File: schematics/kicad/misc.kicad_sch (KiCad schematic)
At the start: 41 parts, among them P4 DIN41612_03x32_C_Split

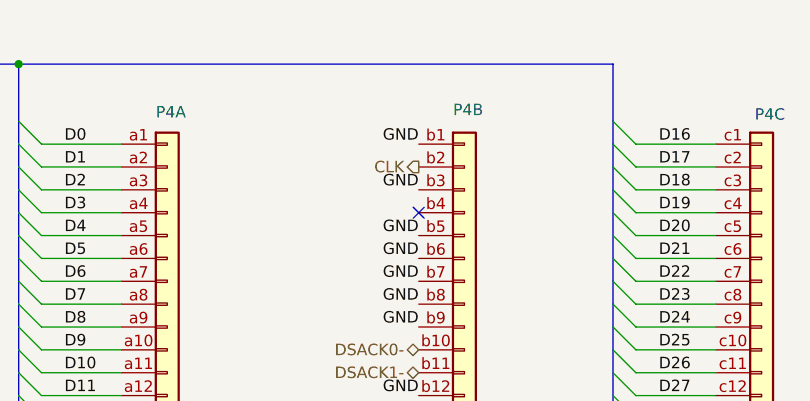
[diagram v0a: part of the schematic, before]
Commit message: Finish routing and misc fixes in the analog section
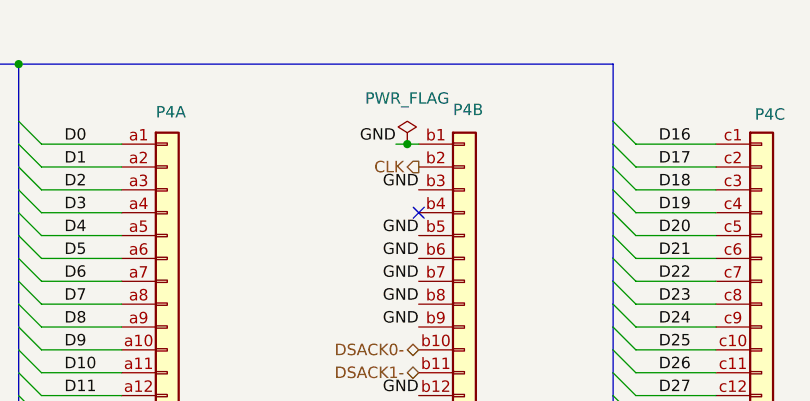
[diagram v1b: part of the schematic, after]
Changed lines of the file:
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@@
 	)
 	(junction
+		(at 208.28 45.72)
+		(diameter 0)
+		(color 0 0 0 0)
+	)
+	(junction
 		(at 73.66 38.1)
 		(diameter 0)
@@
 	(wire
 		(pts
+			(xy 207.01 45.72) (xy 208.28 45.72)
+		)
+		(stroke
+			(width 0)
+			(type default)
+		)
+	)
+	(wire
+		(pts
 			(xy 233.68 63.5) (xy 242.57 63.5)
 		)
@@
 	(wire
 		(pts
+			(xy 208.28 45.72) (xy 209.55 45.72)
+		)
+		(stroke
+			(width 0)
+			(type default)
+		)
+	)
+	(wire
+		(pts
 			(xy 233.68 71.12) (xy 242.57 71.12)
 		)
@@
 	)
 	(label "GND"
-		(at 209.55 45.72 180)
+		(at 207.01 45.72 180)
 		(effects
 			(font
@@
 					(unit 1)
 				)
+			)
+		)
+	)
+	(symbol
+		(lib_id "power:PWR_FLAG")
+		(at 208.28 45.72 0)
+		(unit 1)
+		(exclude_from_sim no)
+		(in_bom yes)
+		(on_board yes)
+		(dnp no)
+		(fields_autoplaced yes)
+		(property "Reference" "#FLG05"
+			(at 208.28 43.815 0)
+			(effects
+				(font
+					(size 1.27 1.27)
+				)
+				(hide yes)
+			)
+		)
+		(property "Value" "PWR_FLAG"
+			(at 208.28 40.64 0)
+			(effects
+				(font
+					(size 1.27 1.27)
+				)
+			)
+		)
+		(property "Footprint" ""
+			(at 208.28 45.72 0)
+			(effects
+				(font
+					(size 1.27 1.27)
+				)
+				(hide yes)
+			)
+		)
+		(property "Datasheet" "~"
+			(at 208.28 45.72 0)
+			(effects
+				(font
+					(size 1.27 1.27)
+				)
+				(hide yes)
+			)
+		)
+		(property "Description" "Special symbol for telling ERC where power comes from"
+			(at 208.28 45.72 0)
+			(effects
+				(font
+					(size 1.27 1.27)
+				)
+				(hide yes)
+			)
+		)
+		(pin "1"
+		)
+		(instances
+			(project "cg4"
+				(path "/7c2b6a13-c303-4adb-8eed-6e6a9ac5307e/1e4cb93f-b1a2-43f5-bc06-3785820075fb"
+					(reference "#FLG05")
+					(unit 1)
+				)
